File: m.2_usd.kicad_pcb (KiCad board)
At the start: 4 copper layers, 22 x 26 mm, 5 parts, among them J1 Bus_M.2_Socket_E, J2 112C-TBAR-R02

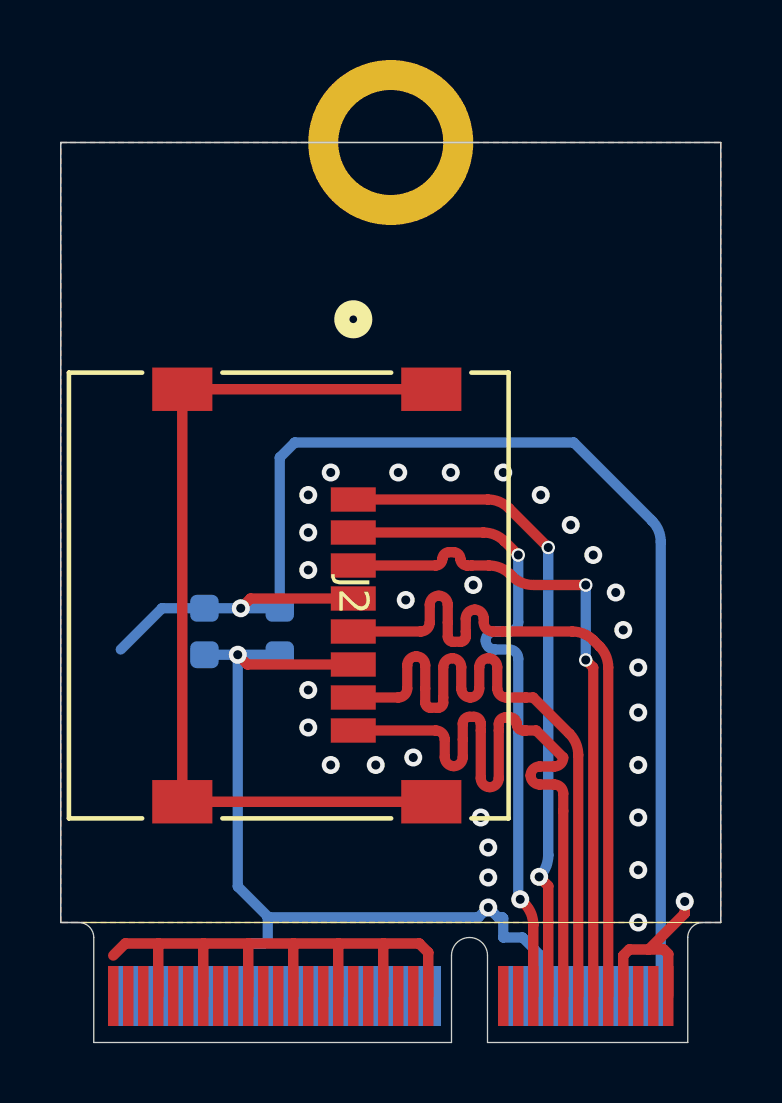
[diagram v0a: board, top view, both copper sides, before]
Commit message: Added extensive via stitching
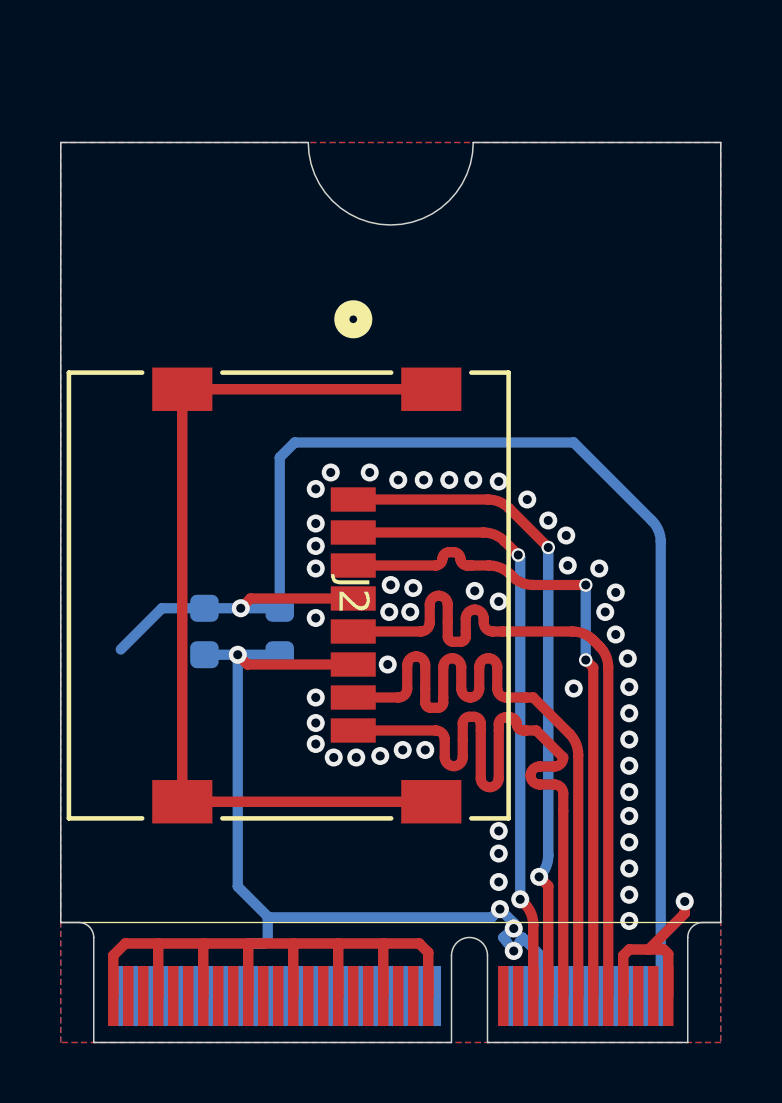
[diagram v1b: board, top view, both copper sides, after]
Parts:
- removed REF**: m2-outer2230, footprints:m2-outer2230
- J1: footprint footprints:m2-padKeyE -> footprints:m2-padKeyE-2230
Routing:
- net GND: track 88.3 -> 90.5 mm, vias 31 -> 55
- net DAT3: track 22.2 -> 20.6 mm
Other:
- board size 22 x 26 mm -> 22 x 30 mm
